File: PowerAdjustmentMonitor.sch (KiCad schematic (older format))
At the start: 19 parts

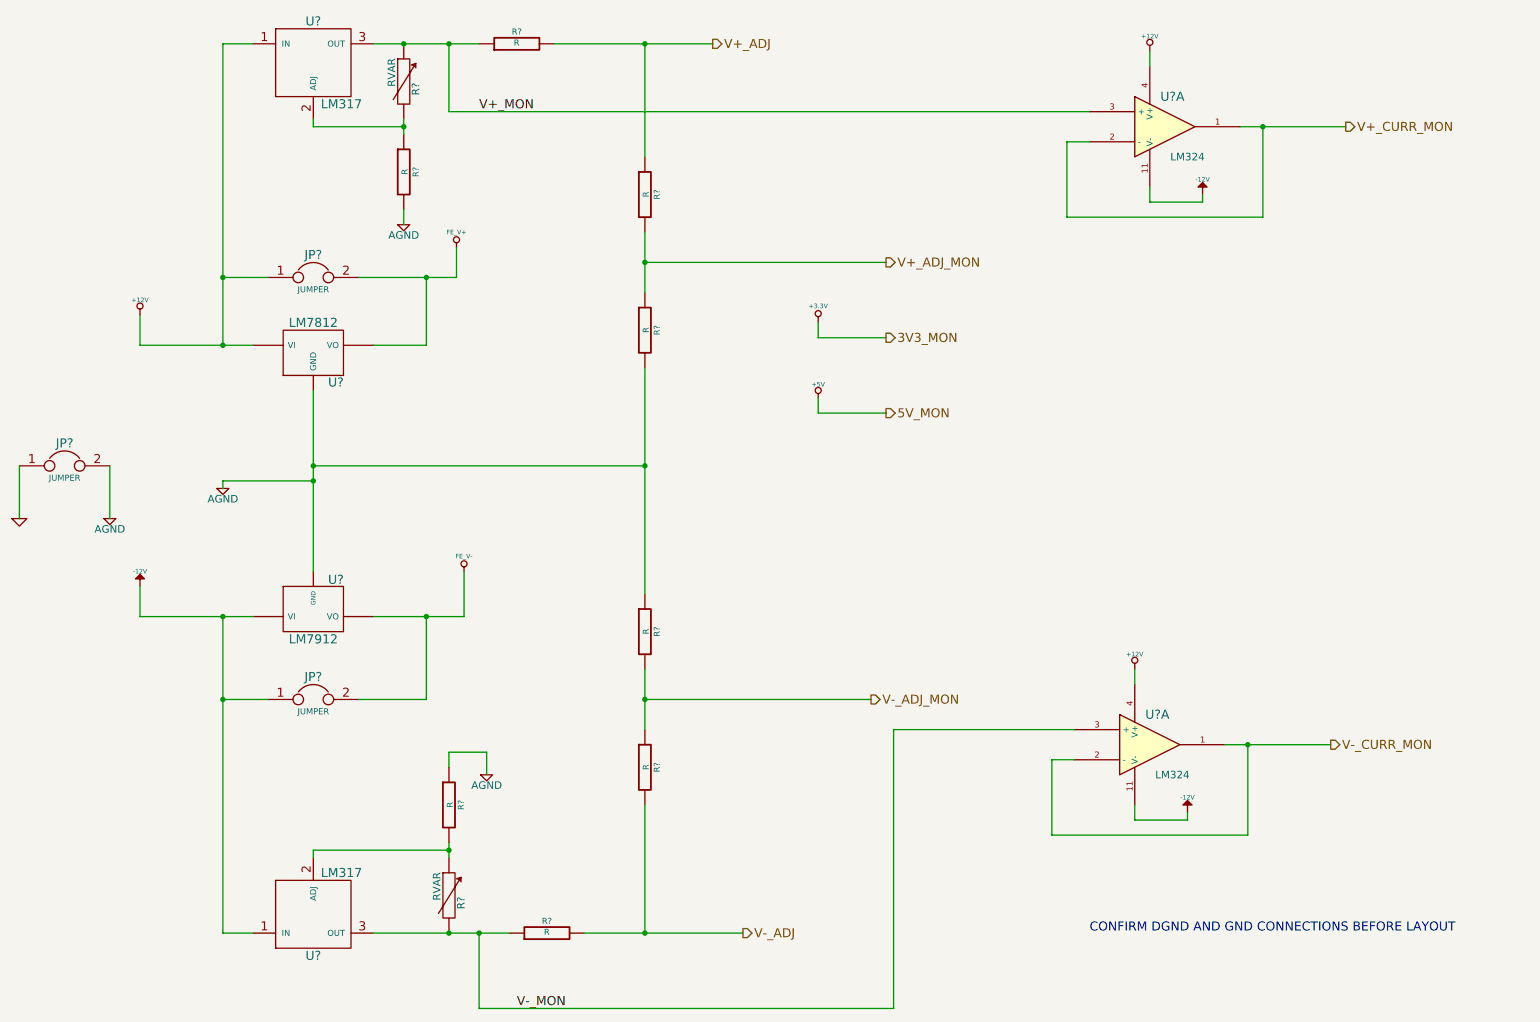
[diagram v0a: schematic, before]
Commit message: Started Layout Outline.  Completed other schem videos
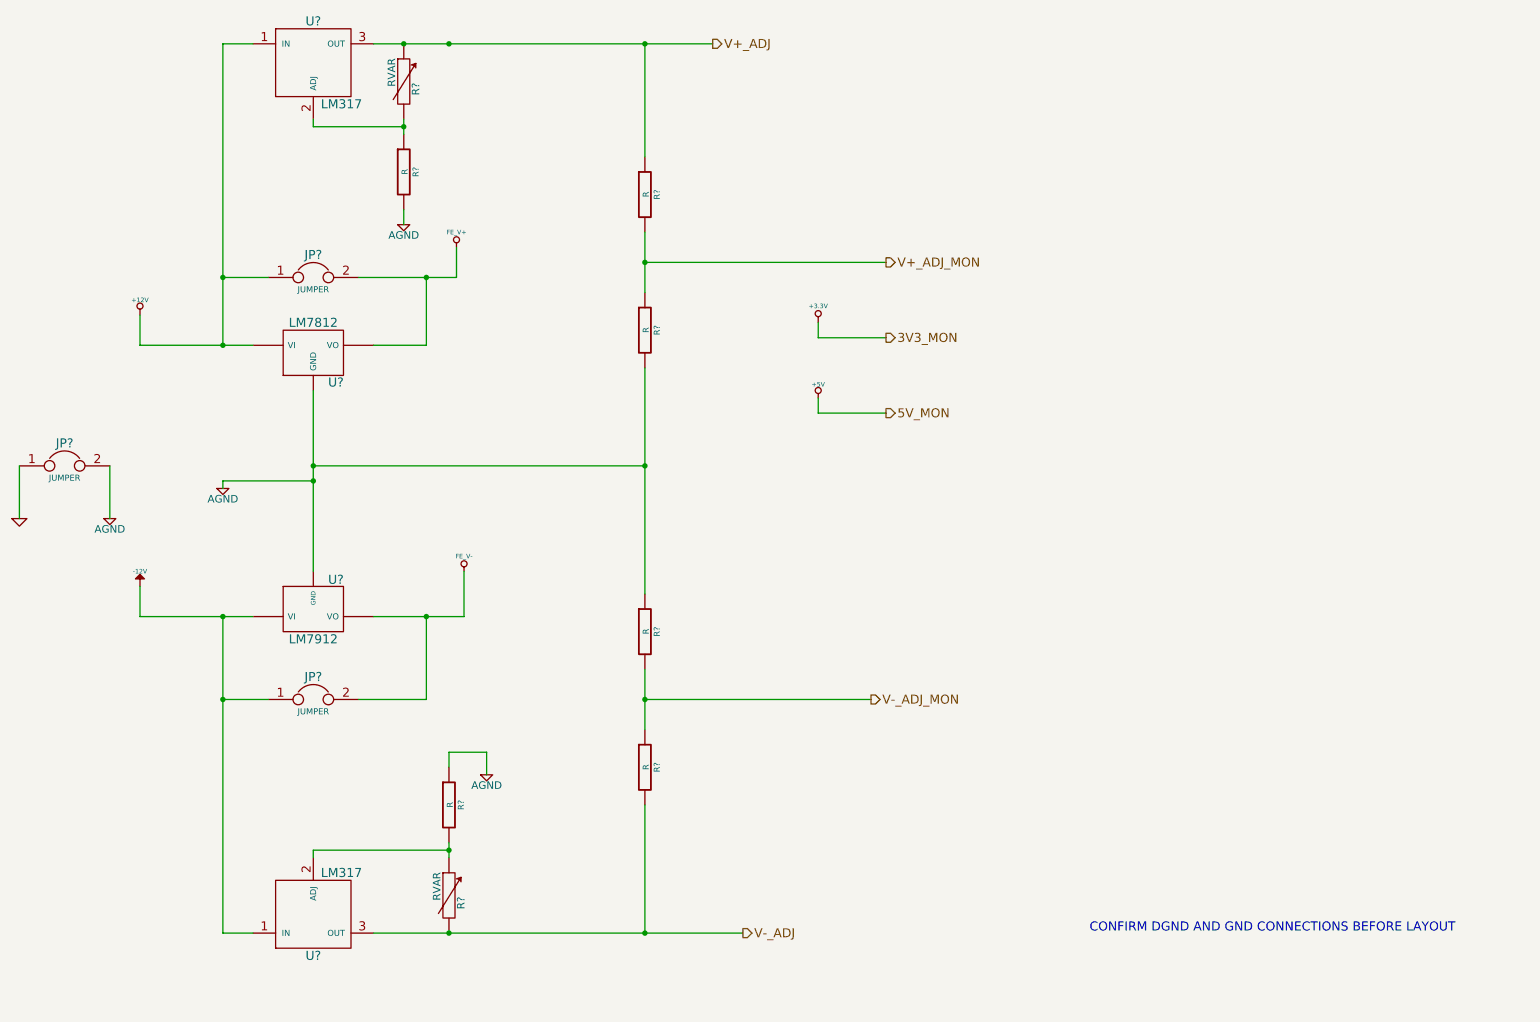
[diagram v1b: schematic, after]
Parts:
- removed R? (x2): R, ~, symbol R
- removed U? (x2): LM324, symbol LM324
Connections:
- net V+_MON is gone; now on net V+_ADJ: R?.1, U?.3 (OUT)
- net V-_MON is gone; now on net V-_ADJ: R?.2, U?.3 (OUT)
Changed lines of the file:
@@
 $Descr A4 11693 8268
 encoding utf-8
-Sheet 9 9
+Sheet 6 9
 Title ""
-Date "11 feb 2014"
+Date "17 feb 2014"
 Rev ""
 Comp ""
@@
 Connection ~ 3650 1650
 Wire Wire Line
-	3450 1100 4150 1100
-Wire Wire Line
-	4650 1100 5700 1100
+	3450 1100 5700 1100
 Connection ~ 3650 1100
 Text HLabel 5700 1100 2    60   Output ~ 0
@@
 Text HLabel 6750 5450 2    60   Output ~ 0
 V-_ADJ_MON
-Text HLabel 9900 1650 2    60   Output ~ 0
-V+_CURR_MON
-Text HLabel 9800 5750 2    60   Output ~ 0
-V-_CURR_MON
 $Comp
 L R R?
@@
 Wire Wire Line
 	6400 3550 6400 3450
-$Comp
-L R R?
-U 1 1 52F83066
-P 4400 1100
-F 0 "R?" V 4480 1100 40  0000 C CNN
-F 1 "R" V 4407 1101 40  0000 C CNN
-F 2 "~" V 4330 1100 30  0000 C CNN
-F 3 "~" H 4400 1100 30  0000 C CNN
-	1    4400 1100
-	0    -1   -1   0
-$EndComp
-$Comp
-L R R?
-U 1 1 52F830FF
-P 4600 7000
-F 0 "R?" V 4680 7000 40  0000 C CNN
-F 1 "R" V 4607 7001 40  0000 C CNN
-F 2 "~" V 4530 7000 30  0000 C CNN
-F 3 "~" H 4600 7000 30  0000 C CNN
-	1    4600 7000
-	0    -1   -1   0
-$EndComp
-Wire Wire Line
-	3450 7000 4350 7000
-Wire Wire Line
-	4850 7000 5900 7000
-Wire Wire Line
-	3950 1100 3950 1550
-Wire Wire Line
-	3950 1550 8200 1550
+Wire Wire Line
+	3450 7000 5900 7000
 Connection ~ 3950 1100
-Text Label 4150 1550 0    60   ~ 0
-V+_MON
-Wire Wire Line
-	4150 7000 4150 7500
-Wire Wire Line
-	4150 7500 6900 7500
-Connection ~ 4150 7000
-Text Label 4400 7500 0    60   ~ 0
-V-_MON
-$Comp
-L LM324 U?
-U 1 1 52F836D4
-P 8700 1650
-F 0 "U?" H 8750 1850 60  0000 C CNN
-F 1 "LM324" H 8850 1450 50  0000 C CNN
-F 2 "" H 8700 1650 60  0000 C CNN
-F 3 "" H 8700 1650 60  0000 C CNN
-	1    8700 1650
-	1    0    0    -1
-$EndComp
-$Comp
-L +12V #PWR?
-U 1 1 52F836ED
-P 8600 1150
-F 0 "#PWR?" H 8600 1100 20  0001 C CNN
-F 1 "+12V" H 8600 1250 30  0000 C CNN
-F 2 "" H 8600 1150 60  0000 C CNN
-F 3 "" H 8600 1150 60  0000 C CNN
-	1    8600 1150
-	1    0    0    -1
-$EndComp
-$Comp
-L -12V #PWR?
-U 1 1 52F836F3
-P 8950 2100
-F 0 "#PWR?" H 8950 2230 20  0001 C CNN
-F 1 "-12V" H 8950 2200 30  0000 C CNN
-F 2 "" H 8950 2100 60  0000 C CNN
-F 3 "" H 8950 2100 60  0000 C CNN
-	1    8950 2100
-	1    0    0    -1
-$EndComp
-Wire Wire Line
-	8200 1750 8050 1750
-Wire Wire Line
-	8050 1750 8050 2250
-Wire Wire Line
-	8050 2250 9350 2250
-Wire Wire Line
-	9350 2250 9350 1650
-Wire Wire Line
-	9200 1650 9900 1650
-Wire Wire Line
-	8600 2050 8600 2150
-Wire Wire Line
-	8600 2150 8950 2150
-Wire Wire Line
-	8950 2150 8950 2100
-Wire Wire Line
-	8600 1250 8600 1150
-Connection ~ 9350 1650
-$Comp
-L LM324 U?
-U 1 1 52F8384E
-P 8600 5750
-F 0 "U?" H 8650 5950 60  0000 C CNN
-F 1 "LM324" H 8750 5550 50  0000 C CNN
-F 2 "" H 8600 5750 60  0000 C CNN
-F 3 "" H 8600 5750 60  0000 C CNN
-	1    8600 5750
-	1    0    0    -1
-$EndComp
-$Comp
-L +12V #PWR?
-U 1 1 52F83854
-P 8500 5250
-F 0 "#PWR?" H 8500 5200 20  0001 C CNN
-F 1 "+12V" H 8500 5350 30  0000 C CNN
-F 2 "" H 8500 5250 60  0000 C CNN
-F 3 "" H 8500 5250 60  0000 C CNN
-	1    8500 5250
-	1    0    0    -1
-$EndComp
-$Comp
-L -12V #PWR?
-U 1 1 52F8385A
-P 8850 6200
-F 0 "#PWR?" H 8850 6330 20  0001 C CNN
-F 1 "-12V" H 8850 6300 30  0000 C CNN
-F 2 "" H 8850 6200 60  0000 C CNN
-F 3 "" H 8850 6200 60  0000 C CNN
-	1    8850 6200
-	1    0    0    -1
-$EndComp
-Wire Wire Line
-	8100 5850 7950 5850
-Wire Wire Line
-	7950 5850 7950 6350
-Wire Wire Line
-	7950 6350 9250 6350
-Wire Wire Line
-	9250 6350 9250 5750
-Wire Wire Line
-	9100 5750 9800 5750
-Wire Wire Line
-	8500 6150 8500 6250
-Wire Wire Line
-	8500 6250 8850 6250
-Wire Wire Line
-	8850 6250 8850 6200
-Wire Wire Line
-	8500 5350 8500 5250
-Connection ~ 9250 5750
-Wire Wire Line
-	6900 7500 6900 5650
-Wire Wire Line
-	6900 5650 8100 5650
 $Comp
 L RVAR R?
